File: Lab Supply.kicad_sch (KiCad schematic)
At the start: 88 parts, among them J1 V+, J2 V-, M1 Fan_4pin, Q1 TIP121, Q2 2N3904, Q3 TIP121, Q5 2N3904, SW1 ENABLE, U1 LM324, U2 LM7812_TO220, U3 MCP4922, U4 LM7805_TO220, U5 LM4040DBZ-2.0, U6 MCP3202

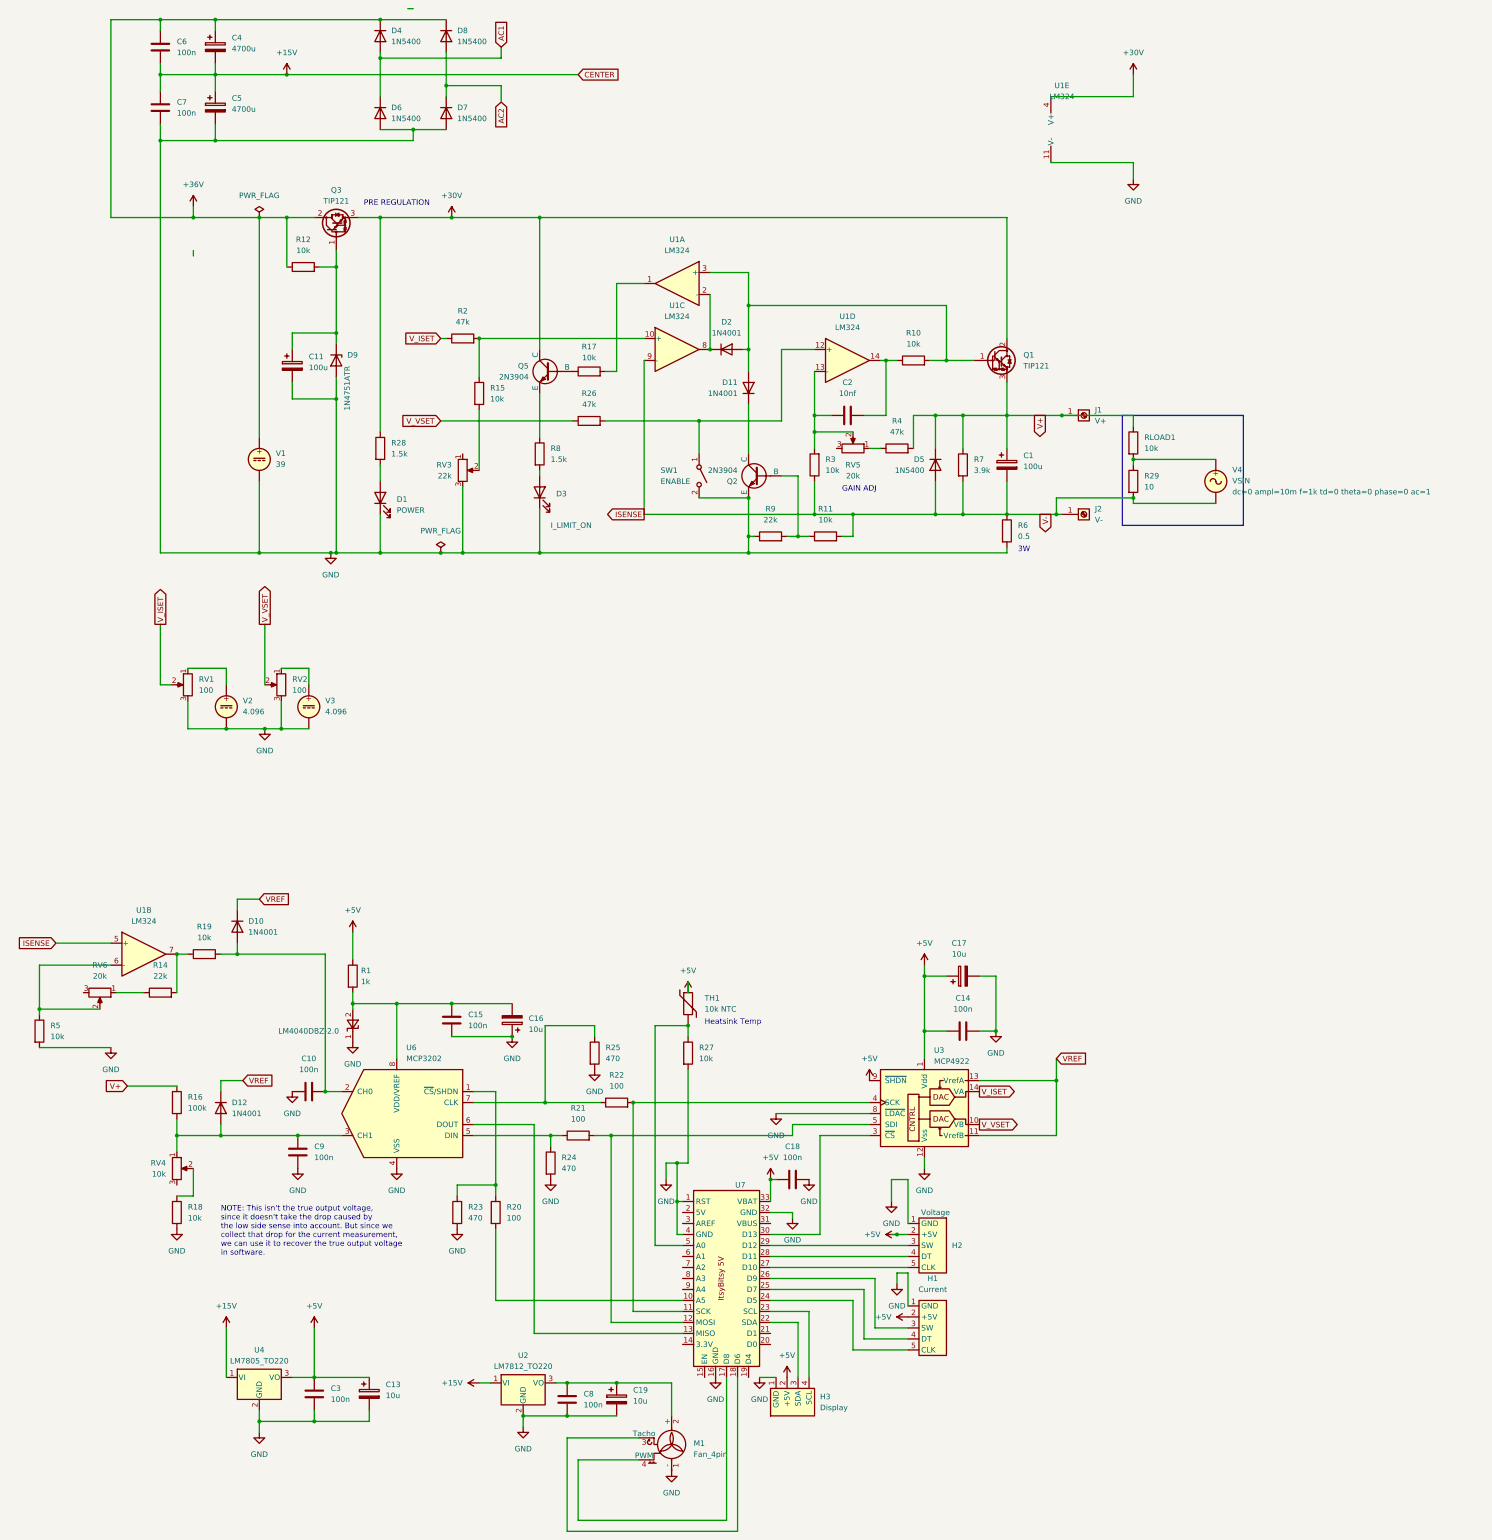
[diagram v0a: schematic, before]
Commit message: WIP
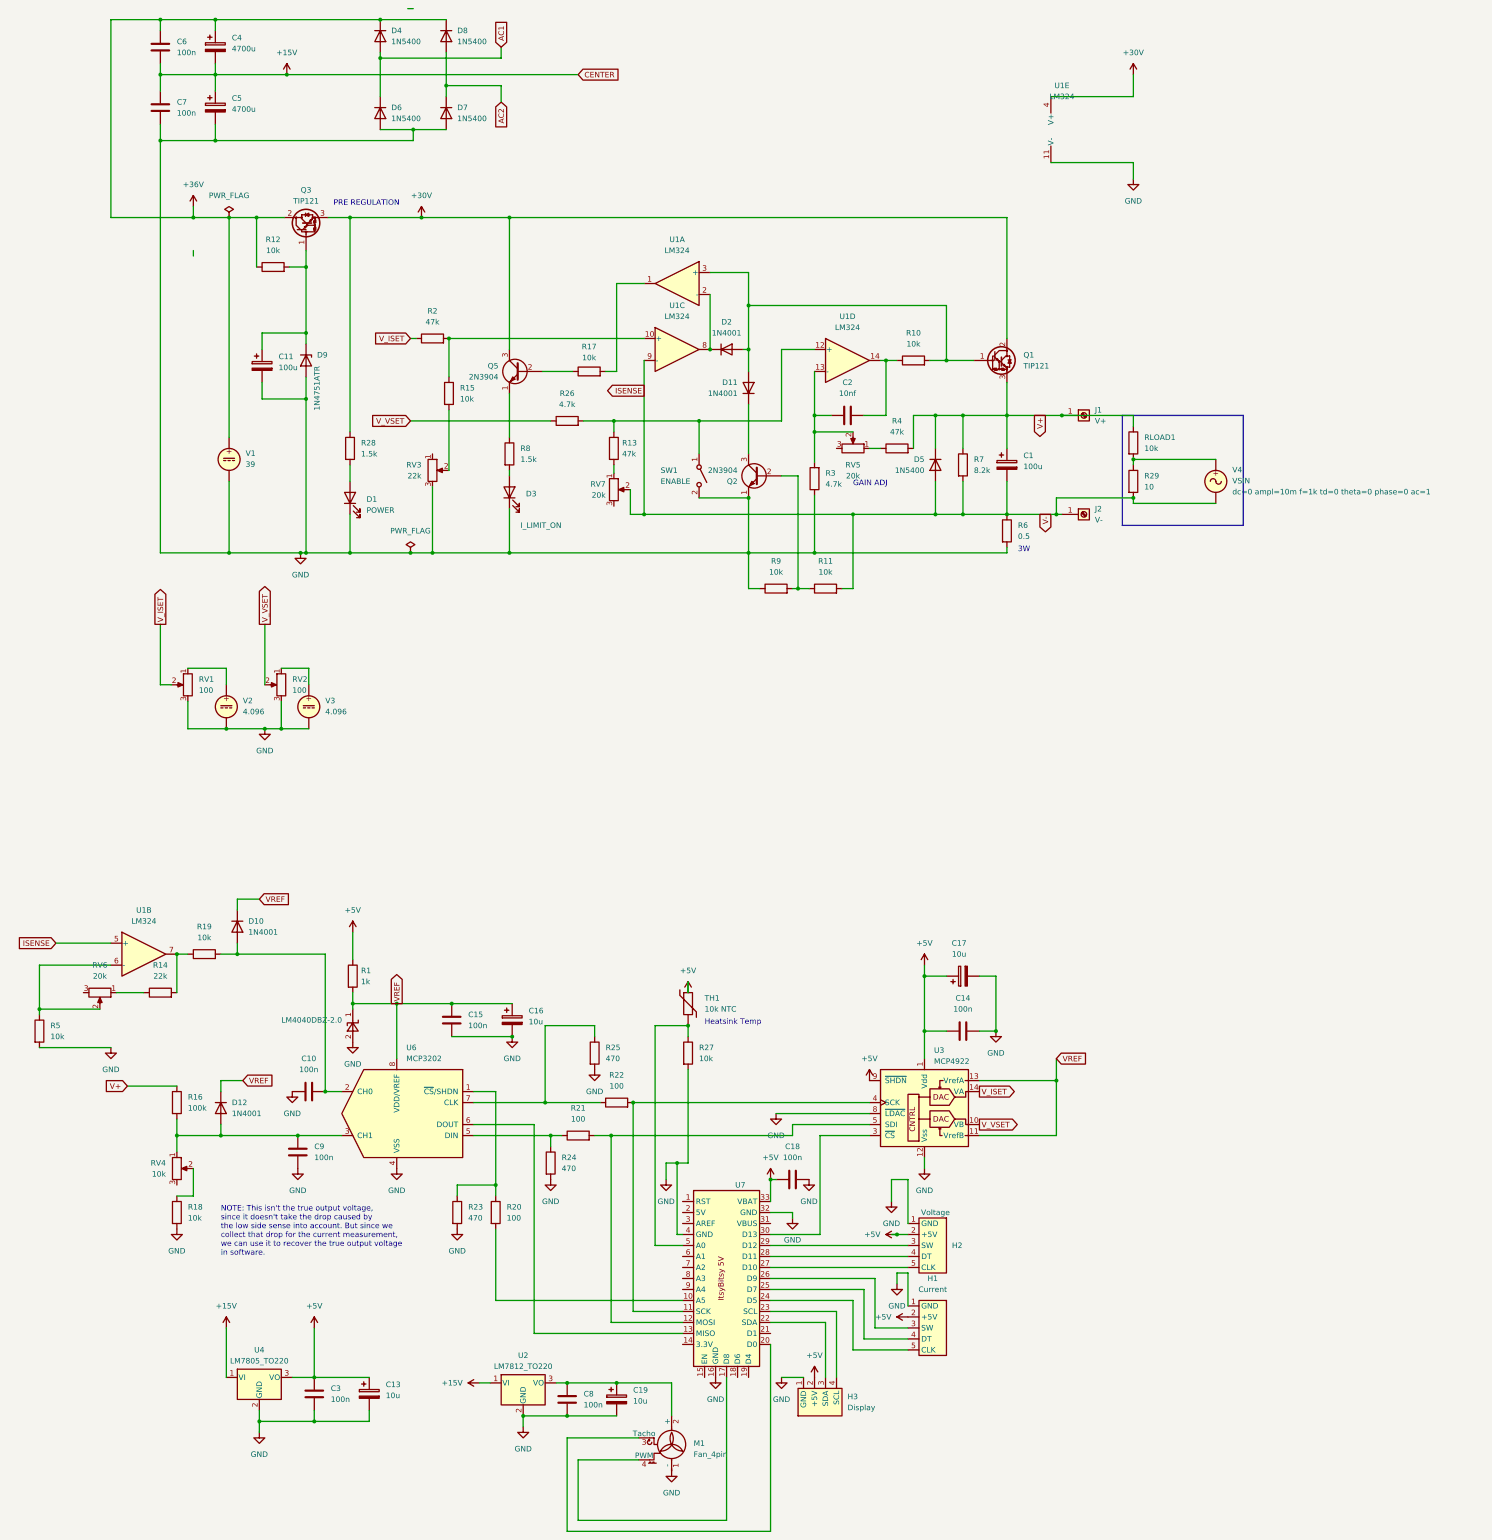
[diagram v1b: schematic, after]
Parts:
- added R13: 47k, symbol Device:R
- added RV7: 20k, symbol Device:R_Potentiometer
- Q2, Q5: footprint Package_TO_SOT_THT:TO-92_HandSolder -> Package_TO_SOT_THT:TO-92_Inline; symbol Simulation_SPICE:NPN -> Transistor_BJT:2N3904
- R26: value 47k -> 4.7k
- R3: value 10k -> 4.7k
- R7: value 3.9k -> 8.2k
- R9: value 22k -> 10k
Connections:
- net +28V: now also Q5.3 (C); no longer Q5.1 (C)
- net GND: now also C16.2, Q2.1 (E), R3.1, U5.2 (A); no longer C16.1, Q2.3 (E), U5.1 (K), U7.1 (RST)
- net ISENSE: now also RV7.2; no longer R3.1
- net VREF: now also C15.1, C16.1, R1.2, U5.1 (K), U6.8 (VDD/VREF)
- net at R26.2, SW1.1 (A), U1.12 (+): now also R13.1
- net at D11.1 (K): now also Q2.3 (C); no longer Q2.1 (C)
- net at M1.3 (Tacho): now also U7.20 (D0); no longer U7.18 (D6)
- net at R8.1: now also Q5.1 (E); no longer Q5.3 (E)
- new net: R13.2, RV7.1
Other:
- moved on the sheet: C11, C16, D1, D3, D9, H3, Q3, R11, R12, R15, R2, R26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
